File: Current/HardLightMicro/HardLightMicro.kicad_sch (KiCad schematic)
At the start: 172 parts, among them J1 USB, K1 Keyswitch, K10 Keyswitch, K11 Keyswitch, K12 Keyswitch, K13 Keyswitch, K14 Keyswitch, K15 Keyswitch, K16 Keyswitch, K17 Keyswitch, K18 Keyswitch, K19 Keyswitch, K2 Keyswitch, K20 Keyswitch, K21 Keyswitch, K22 Keyswitch, K23 Keyswitch, K24 Keyswitch, K25 Keyswitch, K26 Keyswitch, K27 Keyswitch, K28 Keyswitch, K29 Keyswitch, K3 Keyswitch, K30 Keyswitch, K31 Keyswitch, K32 Keyswitch, K33 Keyswitch, K34 Keyswitch, K35 Keyswitch, K36 Keyswitch, K37 Keyswitch, K38 Keyswitch, K39 Keyswitch, K4 Keyswitch, K40 Keyswitch, K41 Keyswitch, K42 Keyswitch, K43 Keyswitch, K44 Keyswitch, K45 Keyswitch, K46 Keyswitch, K47 Keyswitch, K48 Keyswitch, K49 Keyswitch, K5 Keyswitch, K50 Keyswitch, K51 Keyswitch, K52 Keyswitch, K53 Keyswitch, K54 Keyswitch, K55 Keyswitch, K56 Keyswitch, K57 Keyswitch, K58 Keyswitch, K59 Keyswitch, K6 Keyswitch, K60 Keyswitch, K61 Keyswitch, K62 Keyswitch, K63 Keyswitch, K64 Keyswitch, K7 Keyswitch, K8 Keyswitch, K9 Keyswitch, U1 STM32F411CEU6, U2 LDO-3.3, Y1 8MHz

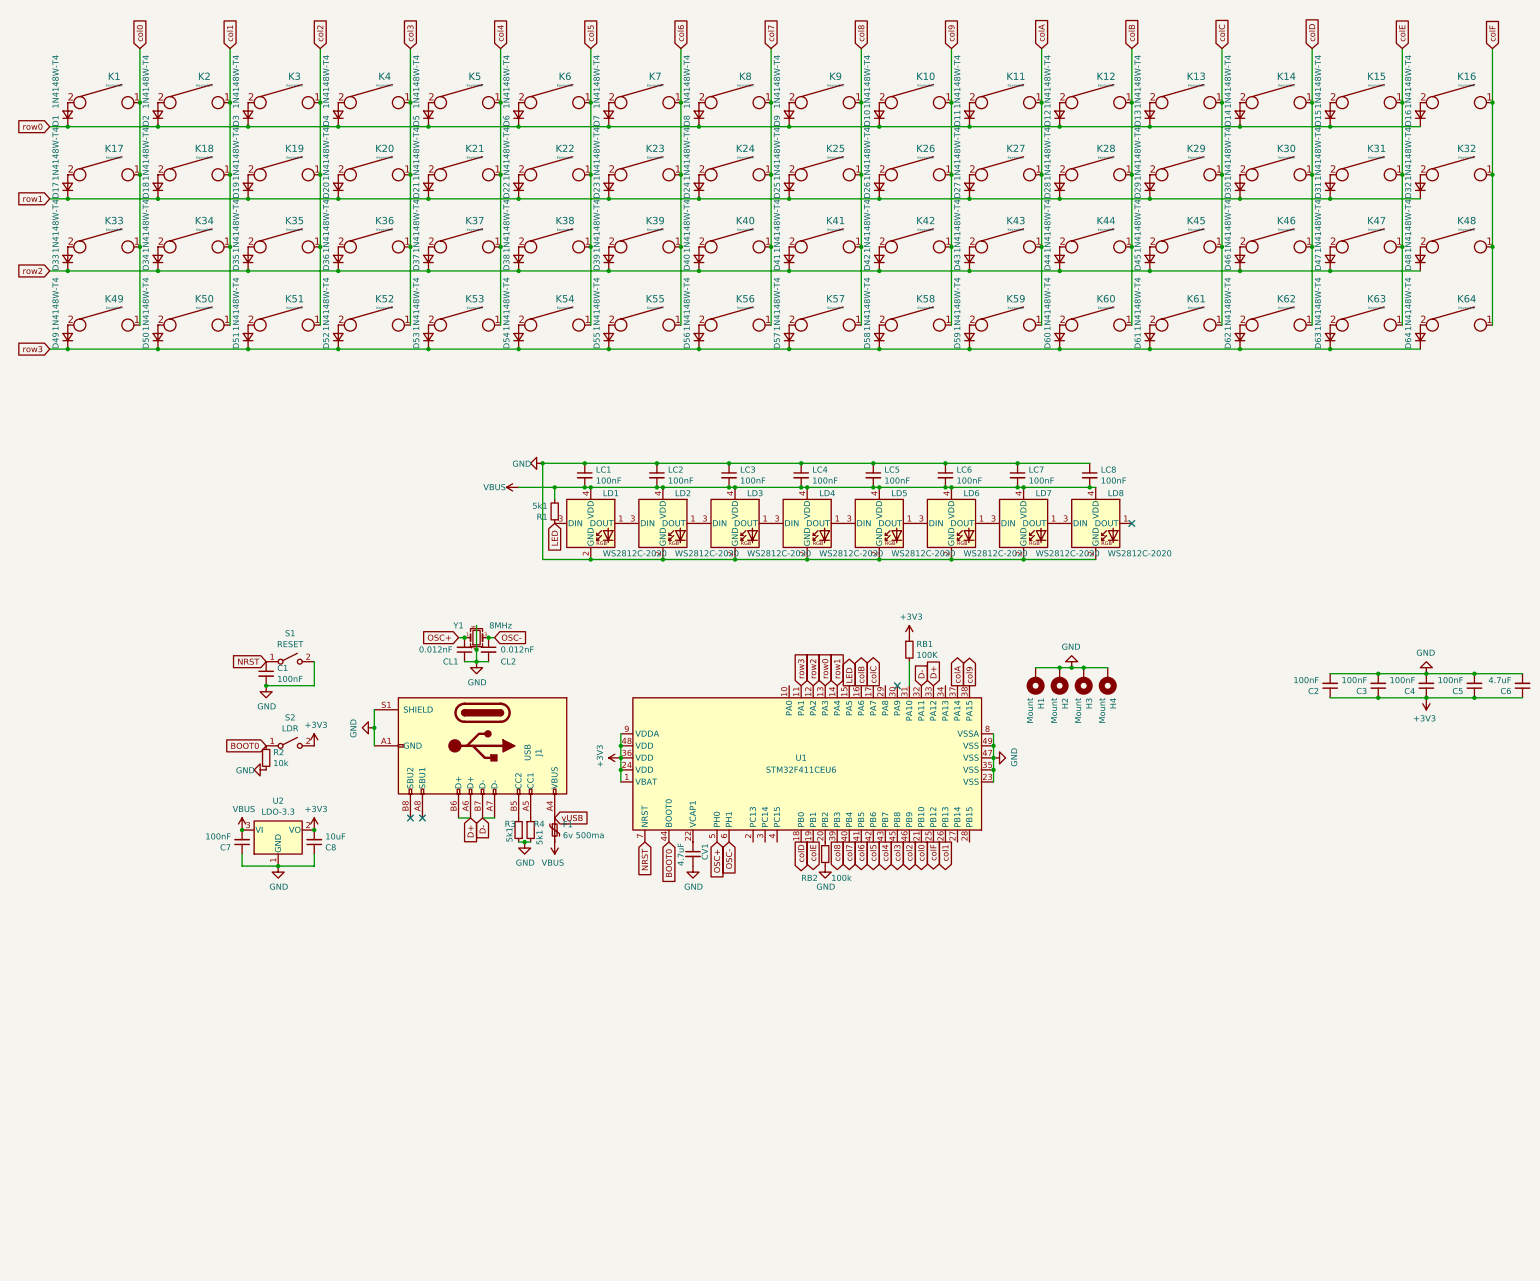
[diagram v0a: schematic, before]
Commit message: Whole bunch of work!
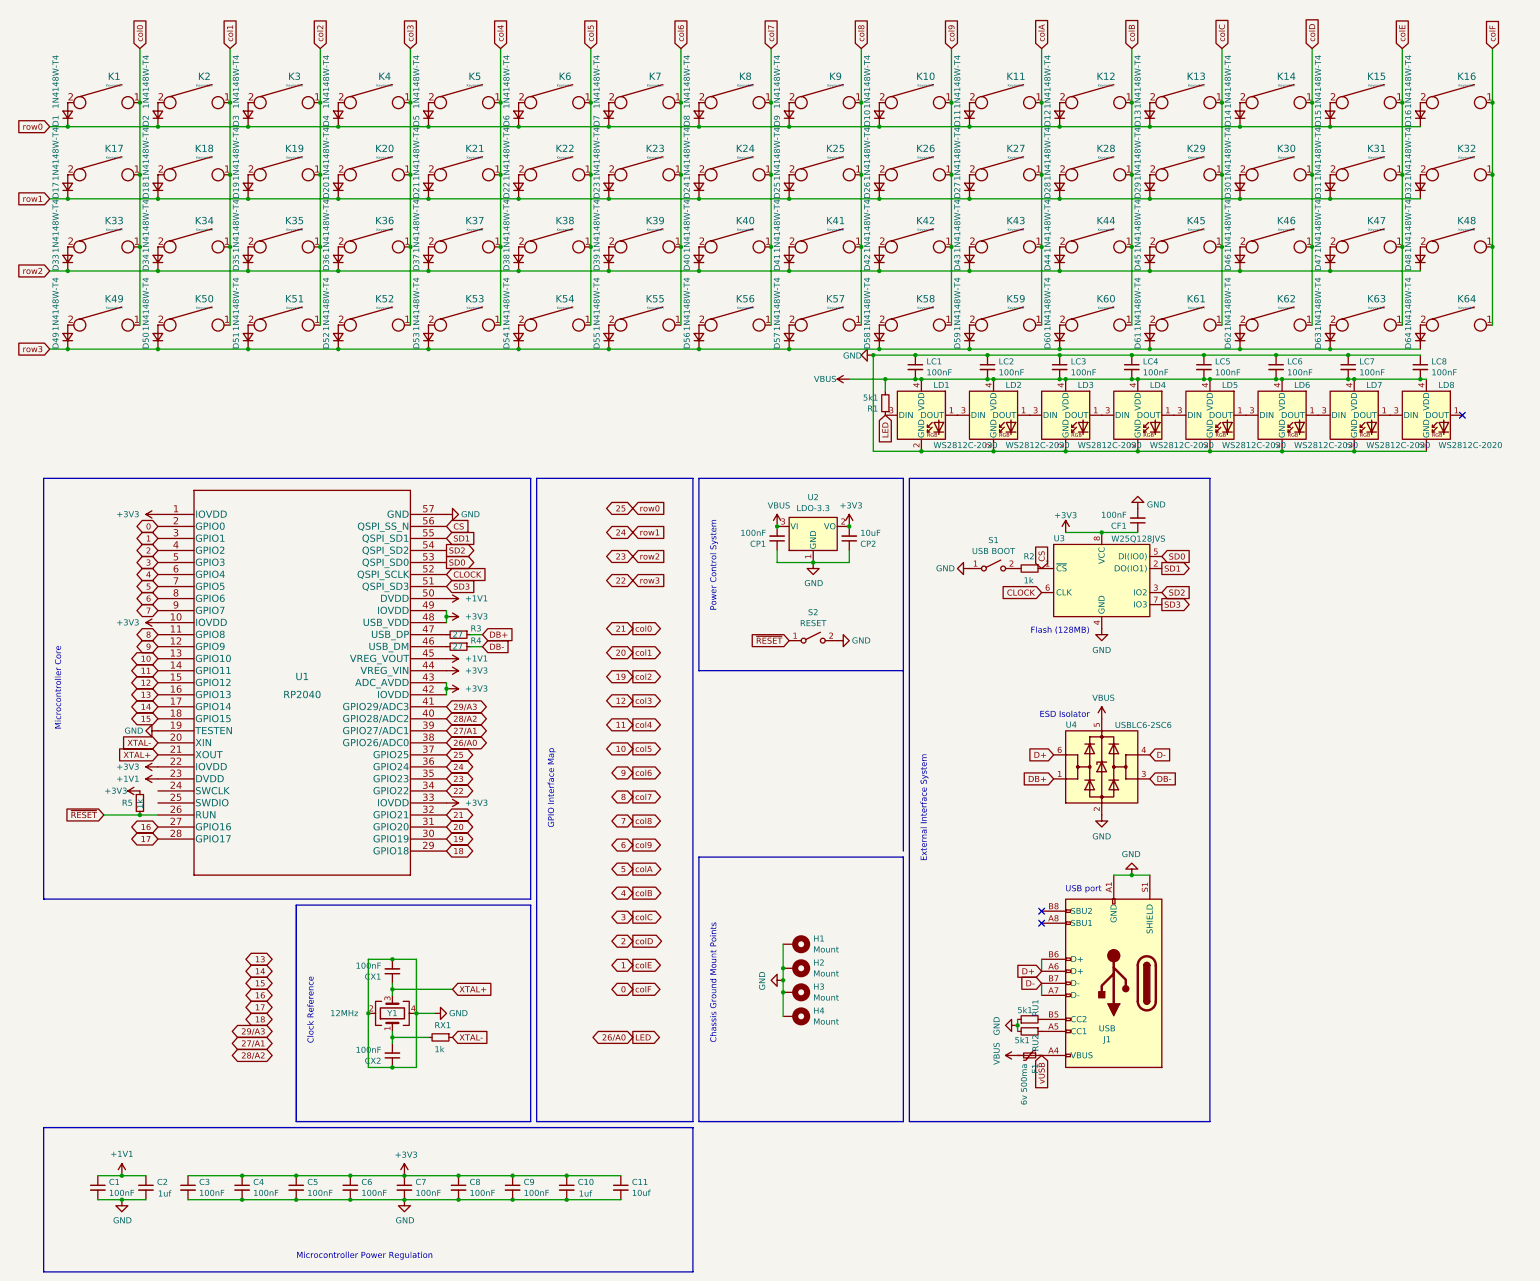
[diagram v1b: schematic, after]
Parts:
- removed CL1, CL2: 0.012nF, EDI:Passive_0402_1005Metric, symbol Device:C_Small
- removed CV1: 4.7uF, EDI:Passive_0402_1005Metric, symbol Device:C_Small
- removed RB1: 100K, EDI:Passive_0402_1005Metric, symbol Device:R_Small
- removed RB2: 100k, EDI:Passive_0402_1005Metric, symbol Device:R_Small
- removed U1: STM32F411CEU6, Package_DFN_QFN:QFN-48-1EP_7x7mm_P0.5mm_EP5.6x5.6mm, symbol MCU_ST_STM32F4:STM32F411CEUx
- removed Y1: 8MHz, Crystal:Crystal_SMD_3225-4Pin_3.2x2.5mm, symbol Device:Crystal_GND24_Small
- added C10: 1uf, EDI:Passive_0402_1005Metric, symbol Device:C_Small
- added C11: 10uf, EDI:Passive_0402_1005Metric, symbol Device:C_Small
- added C9, CF1, CP1, CX1, CX2: 100nF, EDI:Passive_0402_1005Metric, symbol Device:C_Small
- added CP2: 10uF, EDI:Passive_0402_1005Metric, symbol Device:C_Small
- added R5, RX1: 1k, EDI:Passive_0402_1005Metric, symbol Device:R_Small
- added RU1, RU2: 5k1, EDI:Passive_0402_1005Metric, symbol Device:R_Small
- added U1: RP2040, Package_DFN_QFN:QFN-56-1EP_7x7mm_P0.4mm_EP5.6x5.6mm_ThermalVias, symbol RP2040:RP2040
- added U3: W25Q128JVS, Package_SO:SOIC-8_5.23x5.23mm_P1.27mm, symbol Memory_Flash:W25Q128JVS
- added U4: USBLC6-2SC6, Package_TO_SOT_SMD:SOT-23-6, symbol Power_Protection:USBLC6-2SC6
- added Y1: 12MHz, Crystal:Crystal_SMD_3225-4Pin_3.2x2.5mm, symbol Device:Crystal_GND24
- C1, C3, C4, C5, C7: LCSC C307331 -> C1525
- C2: value 100nF -> 1uf; LCSC C307331 -> C52923
- C6: value 4.7uF -> 100nF; LCSC C23733 -> C1525
- C8: value 10uF -> 100nF; LCSC C15525 -> C1525
- F1: footprint Fuse:Fuse_0603_1608Metric_Pad1.05x0.95mm_HandSolder -> Fuse:Fuse_0603_1608Metric
- J1: LCSC C165948 -> C167321
- R2: value 10k -> 1k; LCSC C25744 -> C25905
- R3, R4: value 5k1 -> 27; LCSC C25905 -> C413051
- S1: value RESET -> USB BOOT
- S2: value LDR -> RESET
- renumbered H4 to H1, H3 to H2, H2 to H3, H1 to H4
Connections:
- net +3V3: now also C7.1, C8.1, C10.1, C11.1, C9.1, CF1.1, CP2.2, R5.1, U1.1 (IOVDD), U1.10 (IOVDD), U1.22 (IOVDD), U1.33 (IOVDD), U1.42 (IOVDD), U1.43 (ADC_AVDD), U1.44 (VREG_VIN), U1.48 (USB_VDD), U1.49 (IOVDD), U3.8 (VCC); no longer C2.1, C8.2, S2.2 (B)
- net D+: now also U4.6 (I/O1)
- net D-: now also U4.4 (I/O2)
- net GND: now also C7.2, C8.2, S1.1 (A), S2.2 (B), C10.2, C11.2, C9.2, CF1.2, CP1.1, CP2.1, CX1.2, CX2.1, RU1.1, RU2.2, U1.19 (TESTEN), U1.57 (GND), U3.4 (GND), U4.2 (GND), Y1.2, Y1.4; no longer C7.1, C8.1, R2.2, R3.1, R4.2, S1.2 (B)
- net VBUS: now also CP1.2, U4.5 (VBUS); no longer C7.2
- net at J1.B5 (CC2): now also RU1.2; no longer R3.2
- net at J1.A5 (CC1): now also RU2.1; no longer R4.1
- net BOOT0 renamed CS
- net CS: now also U1.56 (QSPI_SS_N), U3.1 (~{CS}); no longer S2.1 (A)
- net LED renamed 26/A0
- net 26/A0: now also U1.38 (GPIO26/ADC0)
- net NRST renamed +1V1
- net +1V1: now also C2.1, U1.23 (DVDD), U1.45 (VREG_VOUT), U1.50 (DVDD); no longer S1.1 (A)
- net col0 renamed 21
- net 21: now also U1.32 (GPIO21)
- net col1 renamed 20
- net 20: now also U1.31 (GPIO20)
- net col2 renamed 19
- net 19: now also U1.30 (GPIO19)
- net col3 renamed 12
- net 12: now also U1.15 (GPIO12)
- net col4 renamed 11
- net 11: now also U1.14 (GPIO11)
- net col5 renamed 10
- net 10: now also U1.13 (GPIO10)
- net col6 renamed 9
- net 9: now also U1.12 (GPIO9)
- net col7 renamed 8
- net 8: now also U1.11 (GPIO8)
- net col8 renamed 7
- net 7: now also U1.9 (GPIO7)
- net col9 renamed 6
- net 6: now also U1.8 (GPIO6)
- net colA renamed 5
- net 5: now also U1.7 (GPIO5)
- net colB renamed 4
- net 4: now also U1.6 (GPIO4)
- net colC renamed 3
- net 3: now also U1.5 (GPIO3)
- net colD renamed 2
- net 2: now also U1.4 (GPIO2)
- net colE renamed 1
- net 1: now also U1.3 (GPIO1)
- net colF renamed 0
- net 0: now also U1.2 (GPIO0)
- net row0 renamed 25
- net 25: now also U1.37 (GPIO25)
- net row1 renamed 24
- net 24: now also U1.36 (GPIO24)
- net row2 renamed 23
- net 23: now also U1.35 (GPIO23)
- net row3 renamed 22
- net 22: now also U1.34 (GPIO22)
- new net: R2.2, S1.2 (B)
- new net: CX2.2, RX1.2, Y1.1
- new net: R4.2, U1.46 (USB_DM)
- new net: R3.2, U1.47 (USB_DP)
- new net 13: U1.16 (GPIO13)
- new net 14: U1.17 (GPIO14)
- new net 15: U1.18 (GPIO15)
- new net 16: U1.27 (GPIO16)
- new net 17: U1.28 (GPIO17)
- new net 18: U1.29 (GPIO18)
- new net 27/A1: U1.39 (GPIO27/ADC1)
- new net 28/A2: U1.40 (GPIO28/ADC2)
- new net 29/A3: U1.41 (GPIO29/ADC3)
- new net CLOCK: U1.52 (QSPI_SCLK), U3.6 (CLK)
- new net DB+: R3.1, U4.1 (I/O1)
- new net DB-: R4.1, U4.3 (I/O2)
- new net SD0: U1.53 (QSPI_SD0), U3.5 (DI(IO0))
- new net SD1: U1.55 (QSPI_SD1), U3.2 (DO(IO1))
- new net SD2: U1.54 (QSPI_SD2), U3.3 (IO2)
- new net SD3: U1.51 (QSPI_SD3), U3.7 (IO3)
- new net XTAL+: CX1.1, U1.21 (XOUT), Y1.3
- new net XTAL-: RX1.1, U1.20 (XIN)
- new net ~{RESET}: R5.2, S2.1 (A), U1.26 (RUN)
- no-connect marks 4 -> 3
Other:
- note added: "Chassis Ground Mount Points"
- note added: "Clock Reference"
- note added: "ESD Isolator"
- note added: "External Interface System"
- note added: "Flash (128MB)"
- note added: "GPIO Interface Map"
- note added: "Microcontroller Core"
- note added: "Microcontroller Power Regulation"
- note added: "Power Control System"
- note added: "USB port"
- moved on the sheet: H1, H2, H3, H4, LC1, LC2, LC3, LC4, LC5, LC6, LC7, LC8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
